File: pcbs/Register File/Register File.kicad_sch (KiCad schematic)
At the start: 0 parts

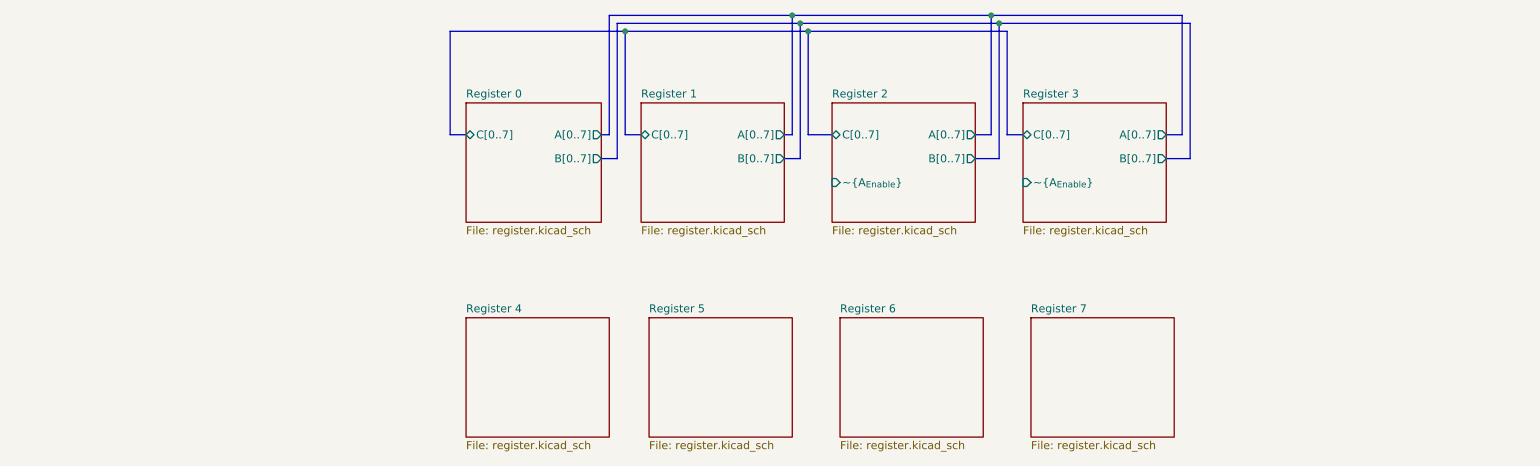
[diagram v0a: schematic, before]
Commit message: More work
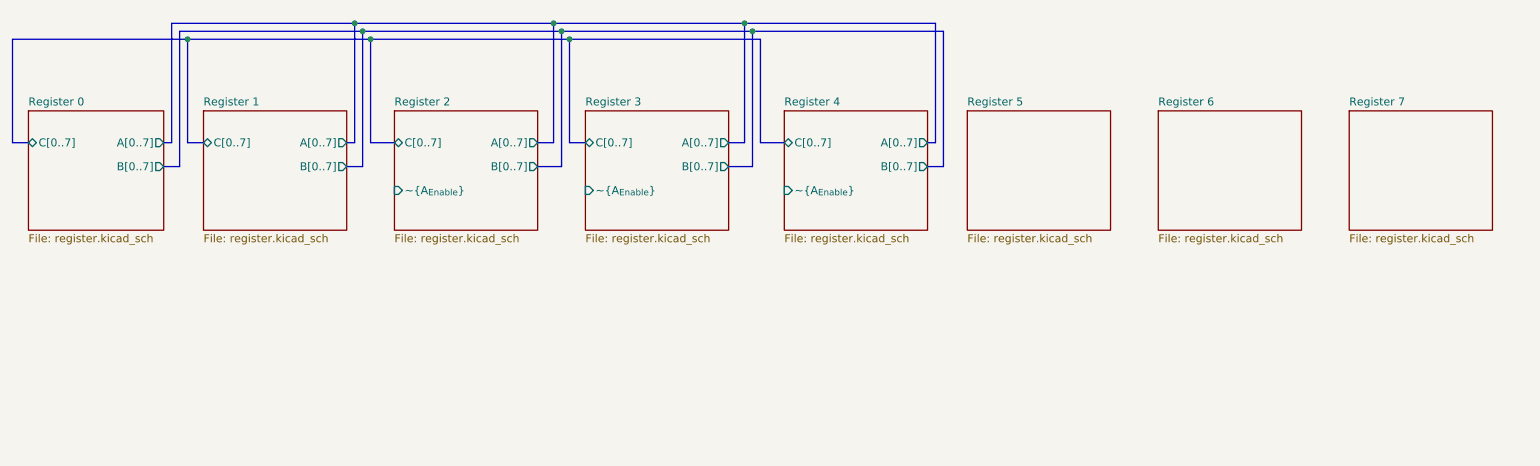
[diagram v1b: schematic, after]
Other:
- sheet Register 4 ports: added A[0..7], B[0..7], C[0..7], ~{A_{Enable}}; removed none
